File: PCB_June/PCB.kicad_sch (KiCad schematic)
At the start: 25 parts, among them J201 FH34SRJ-24S-0.5SH_99_, Q201 BSS138, Q202 S8050, U203 AO3401

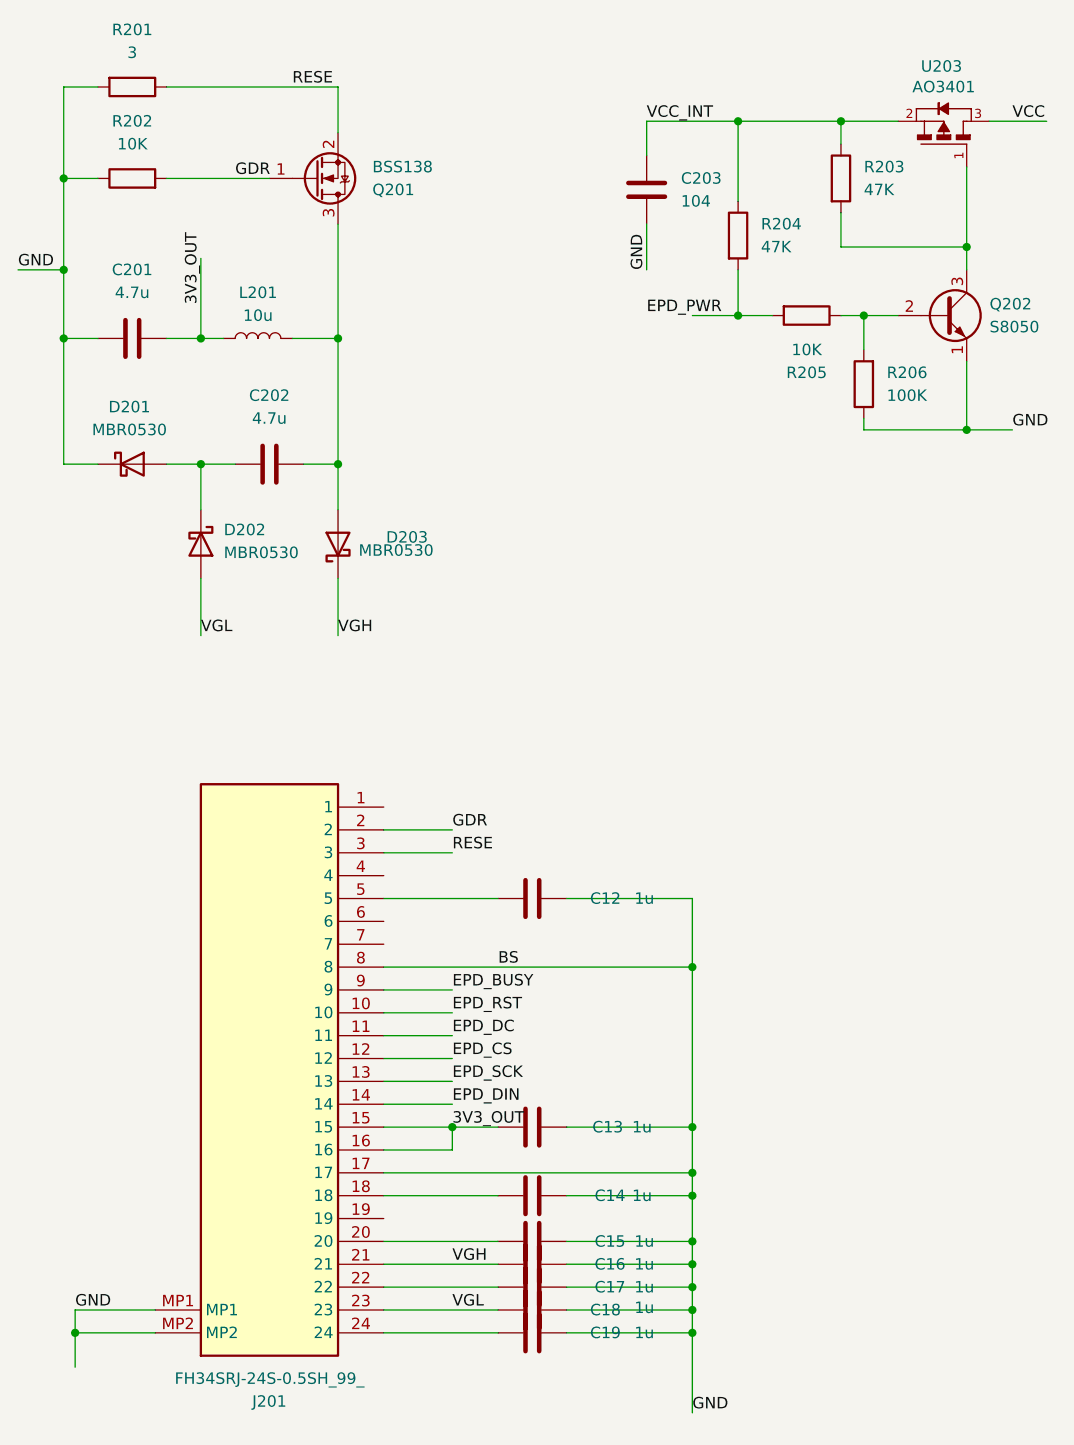
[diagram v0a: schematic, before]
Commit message: hhhhh
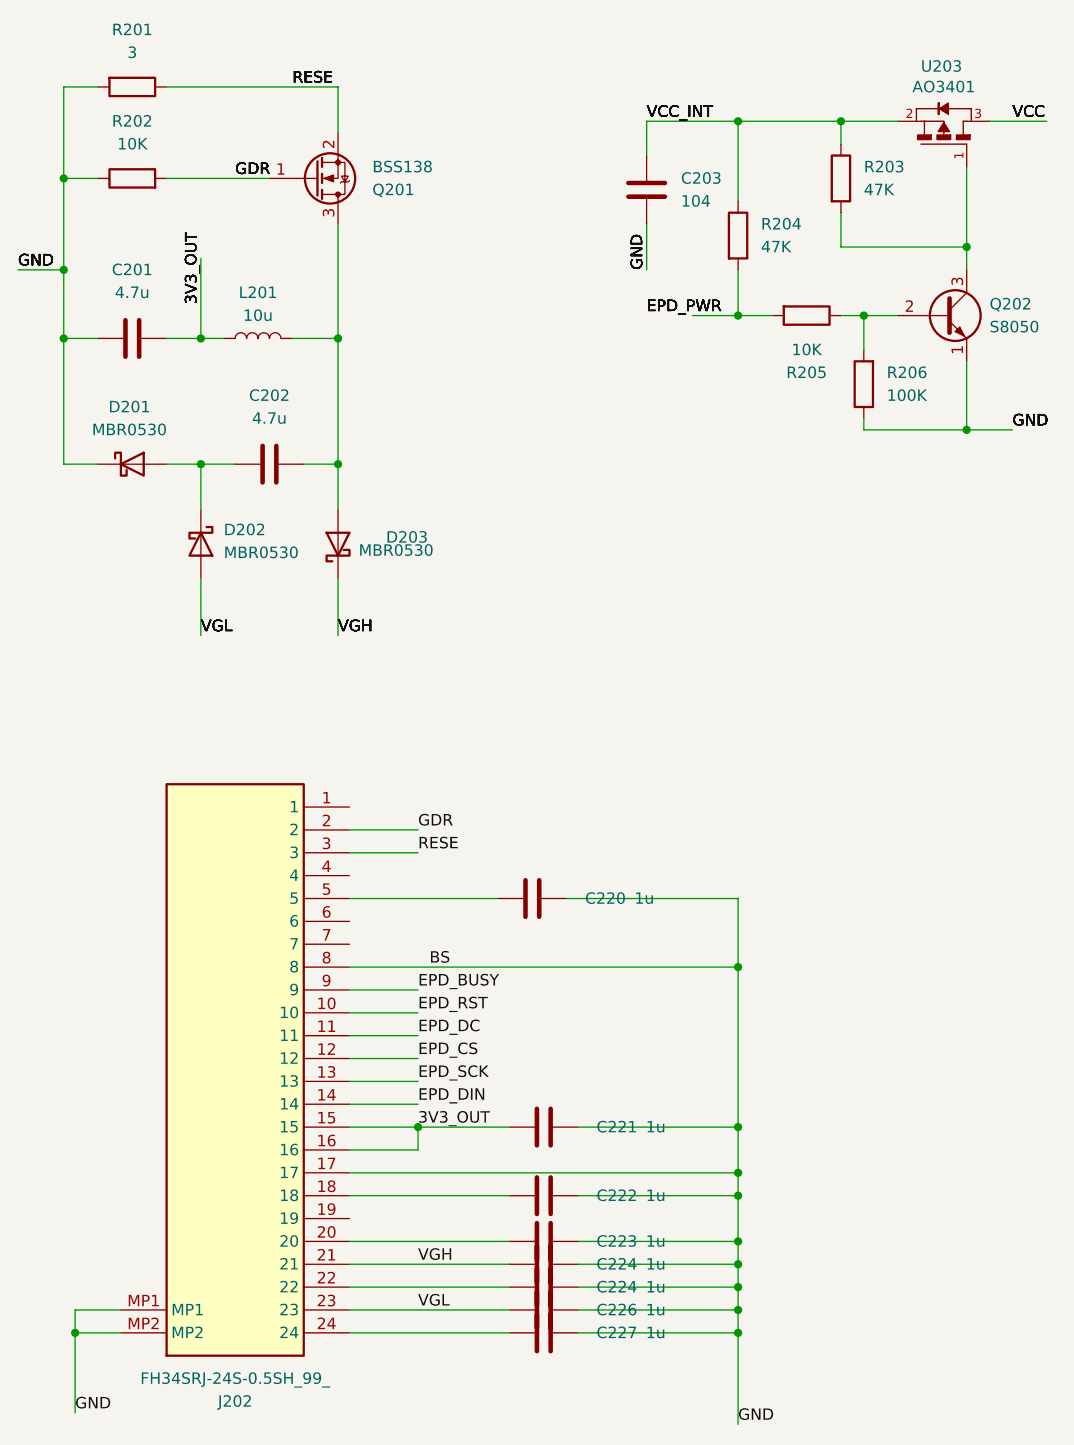
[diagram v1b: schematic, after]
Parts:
- removed C12, C13, C14, C15, C16, C17, C18, C19: 1u, Capacitor_SMD:C_0805_2012Metric_Pad1.18x1.45mm_HandSolder, symbol Device:C
- removed J201: FH34SRJ-24S-0.5SH_99_, Custom:FH34SRJ24S05SH99, symbol FH34SRJ-24S-0.5SH(99):FH34SRJ-24S-0.5SH_99_
- added C220, C221, C222, C223, C224 (x2), C226, C227: 1u, Capacitor_SMD:C_0805_2012Metric_Pad1.18x1.45mm_HandSolder, symbol Device:C
- added J202: FH34SRJ-24S-0.5SH_99_, Custom:FH34SRJ24S05SH99, symbol FH34SRJ-24S-0.5SH(99):FH34SRJ-24S-0.5SH_99_
- Q202: footprint Package_TO_SOT_SMD:SOT-23-3 -> Package_TO_SOT_THT:TO-92_Inline
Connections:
- net 3V3_OUT: now also C221.1, J202.15, J202.16
- net BS: now also C220.2, C221.2, C222.2, C223.2, C224.2, C224.2, C226.2, C227.2, J202.17, J202.8, J202.MP1, J202.MP2
- net EPD_BUSY: now also J202.9
- net EPD_CS: now also J202.12
- net EPD_DC: now also J202.11
- net EPD_DIN: now also J202.14
- net EPD_RST: now also J202.10
- net EPD_SCK: now also J202.13
- net GDR: now also J202.2
- net RESE: now also J202.3
- net VGH: now also C224.1, J202.21
- net VGL: now also C226.1, J202.23
- new net: C222.1, J202.18
- new net: C223.1, J202.20
- new net: C224.1, J202.22
- new net: C227.1, J202.24
- new net: C220.1, J202.5
